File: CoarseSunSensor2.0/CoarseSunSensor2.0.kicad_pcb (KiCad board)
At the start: 2 copper layers, 45.4 x 14.2 mm, 23 parts, among them IC1 ADS1115IDGSR, J1 53261-0571

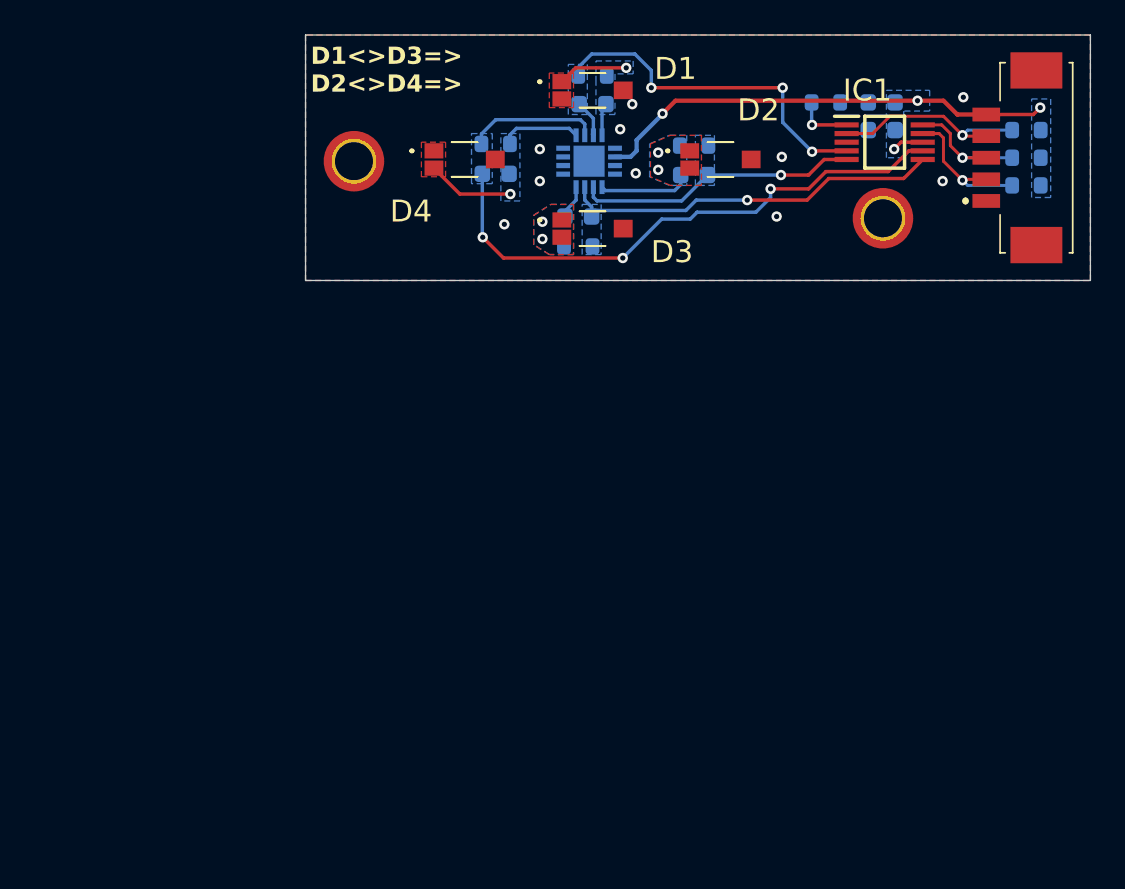
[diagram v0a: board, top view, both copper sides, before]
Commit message: Board repositioning
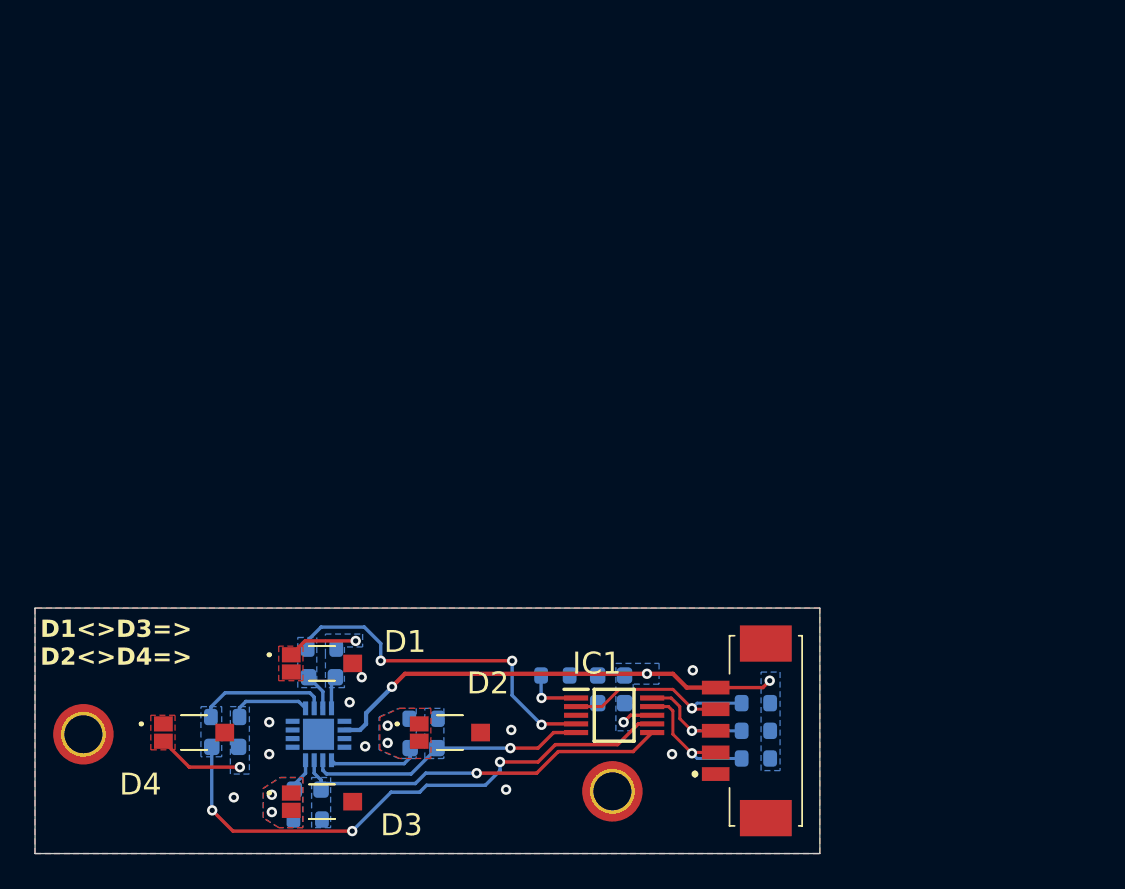
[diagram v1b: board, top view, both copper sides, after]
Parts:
- moved C1 36.7 mm to (137.8, 97.2)
- moved C2 36.7 mm to (143.6, 101.2)
- moved C4 36.7 mm to (132.2, 101.2)
- moved C6 36.7 mm to (154.5, 98.7)
- moved J1 36.7 mm to (161.3, 100.2)
- moved R4 36.7 mm to (132.2, 99.5)
- moved R6 36.7 mm to (162.8, 98.7)
- moved R8 36.7 mm to (162.8, 100.2)
- moved C5 36.7 mm to (154.5, 97.0)
- moved H1 36.7 mm to (124.0, 100.5)
- moved R1 36.7 mm to (137.8, 95.5)
- moved R5 36.7 mm to (151.2, 97.0)
- moved C3 36.7 mm to (136.9, 103.7)
- moved H2 36.7 mm to (154.6, 103.8)
- moved U1 36.7 mm to (137.6, 100.5)
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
